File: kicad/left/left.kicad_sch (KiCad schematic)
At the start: 48 parts, among them J1 59453-121110ECHLF, J2 59453-051110ECHLF, J3 59453-051110ECHLF, J4 59453-081110EDHLF, J5 59453-081110EDHLF, U1 RP2040_Zero

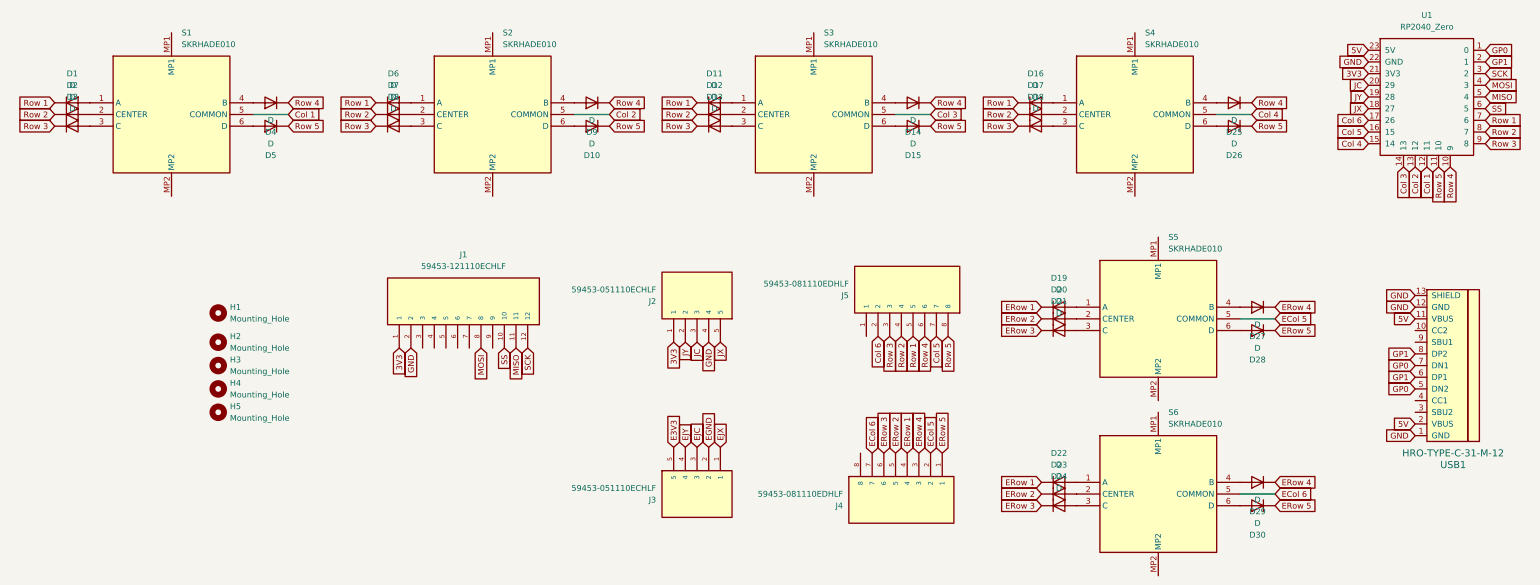
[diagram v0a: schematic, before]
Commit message: break up parts
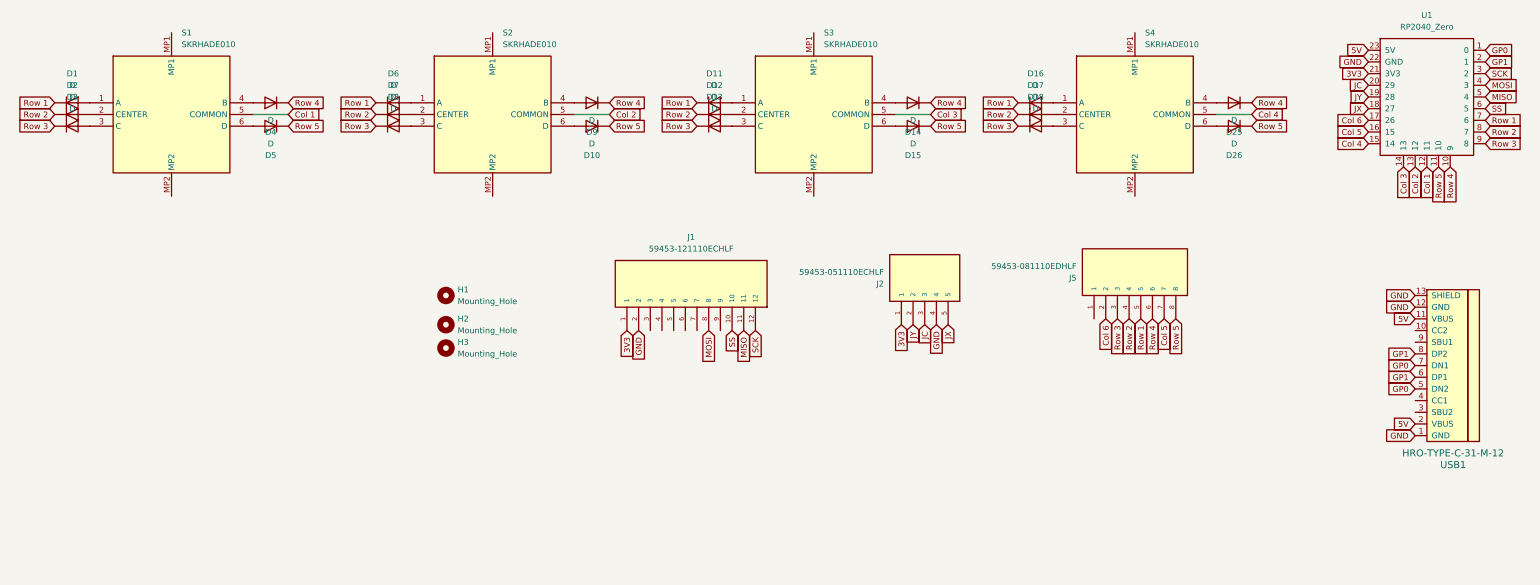
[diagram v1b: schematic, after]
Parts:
- removed D19, D20, D21, D22, D23, D24, D27, D28, D29, D30: D, ScottoKeebs_Components:Diode_SOD-123, symbol Device:D
- removed H4, H5: Mounting_Hole, MountingHole:MountingHole_2.2mm_M2_Pad_Via, symbol ScottoKeebs:Placeholder_Mounting_Hole
- removed J3: 59453-051110ECHLF, AMPHENOL_59453-051110ECHLF, symbol 59453-051110ECHLF:59453-051110ECHLF
- removed J4: 59453-081110EDHLF, AMPHENOL_59453-081110EDHLF, symbol 59453-081110EDHLF:59453-081110EDHLF
- removed S5, S6: SKRHADE010, SKRHADE010, symbol SKRHADE010:SKRHADE010
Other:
- moved on the sheet: H1, H2, H3, J1, J2, J5

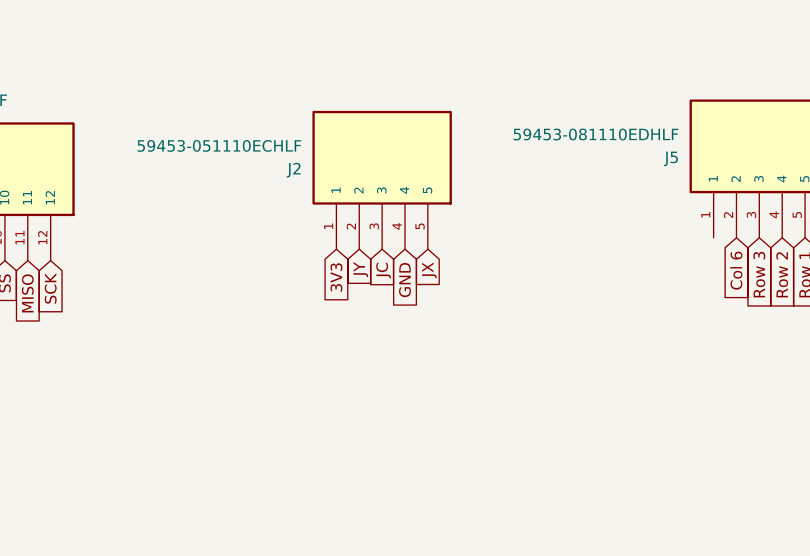
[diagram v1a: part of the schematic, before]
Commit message: wiring
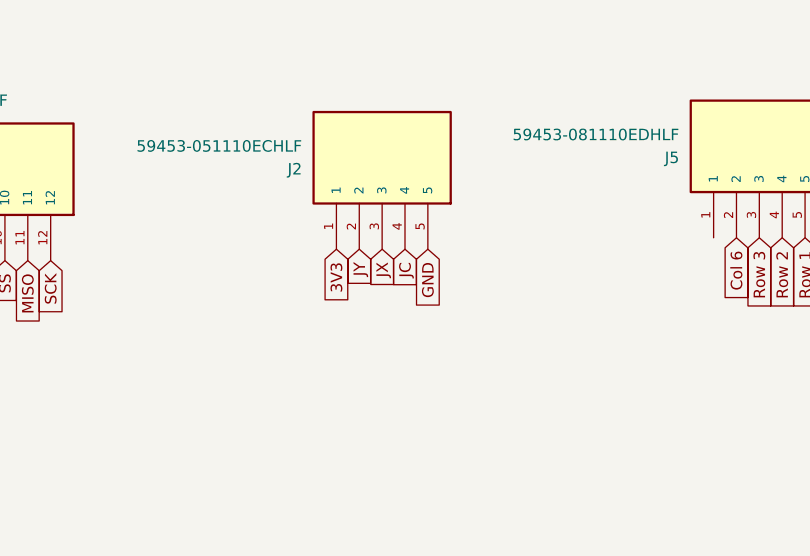
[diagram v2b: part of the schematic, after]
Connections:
- net GND: now also J2.5; no longer J2.4
- net JC: now also J2.4; no longer J2.3
- net JX: now also J2.3; no longer J2.5

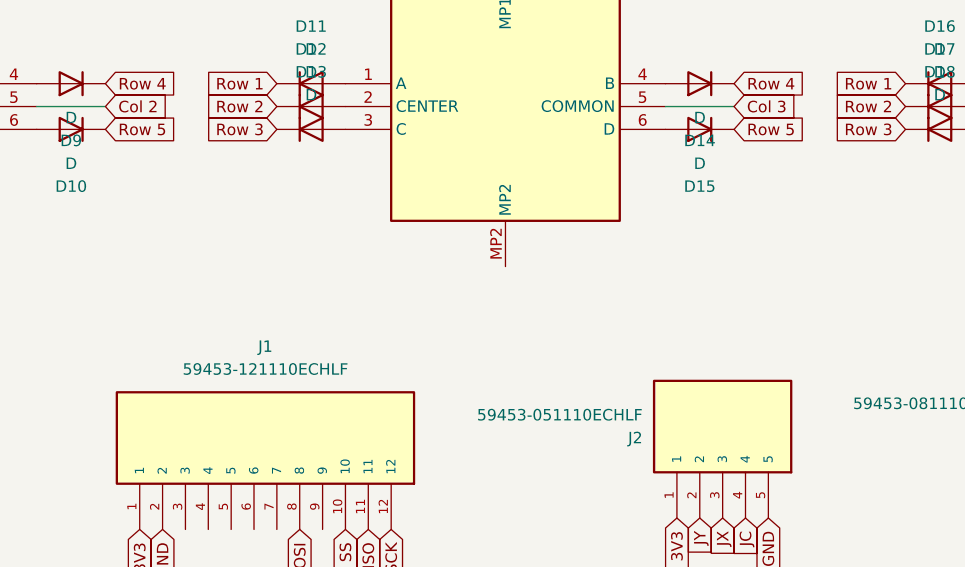
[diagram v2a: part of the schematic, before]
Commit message: Add connectors
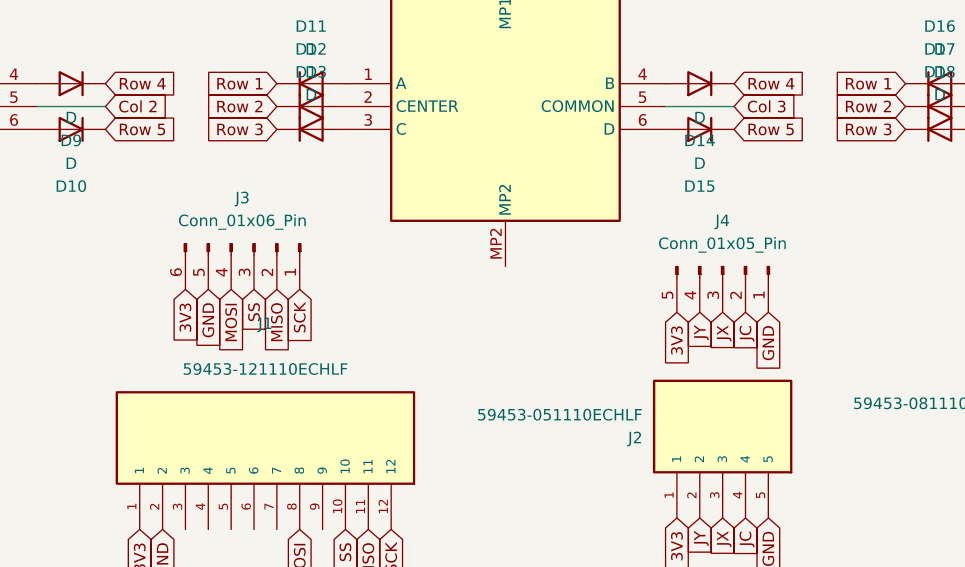
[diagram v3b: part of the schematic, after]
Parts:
- added J3: Conn_01x06_Pin, footprints:Pointing-connector, symbol Connector:Conn_01x06_Pin
- added J4: Conn_01x05_Pin, footprints:Joystick-connector, symbol Connector:Conn_01x05_Pin
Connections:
- net 3V3: now also J3.6 (Pin_6), J4.5 (Pin_5)
- net GND: now also J3.5 (Pin_5), J4.1 (Pin_1)
- net JC: now also J4.2 (Pin_2)
- net JX: now also J4.3 (Pin_3)
- net JY: now also J4.4 (Pin_4)
- net MISO: now also J3.2 (Pin_2)
- net MOSI: now also J3.4 (Pin_4)
- net SCK: now also J3.1 (Pin_1)
- net SS: now also J3.3 (Pin_3)
